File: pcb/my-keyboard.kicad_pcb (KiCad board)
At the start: 2 copper layers, 8 parts, among them J1 Conn_01x04_Socket, SW1 SW_Push, SW2 SW_Push, SW3 SW_Push, SW4 SW_Push, SW5 RotaryEncoder_Switch, SW6 RotaryEncoder_Switch, U1 MOUDLE-SEEEDUINO-XIAO

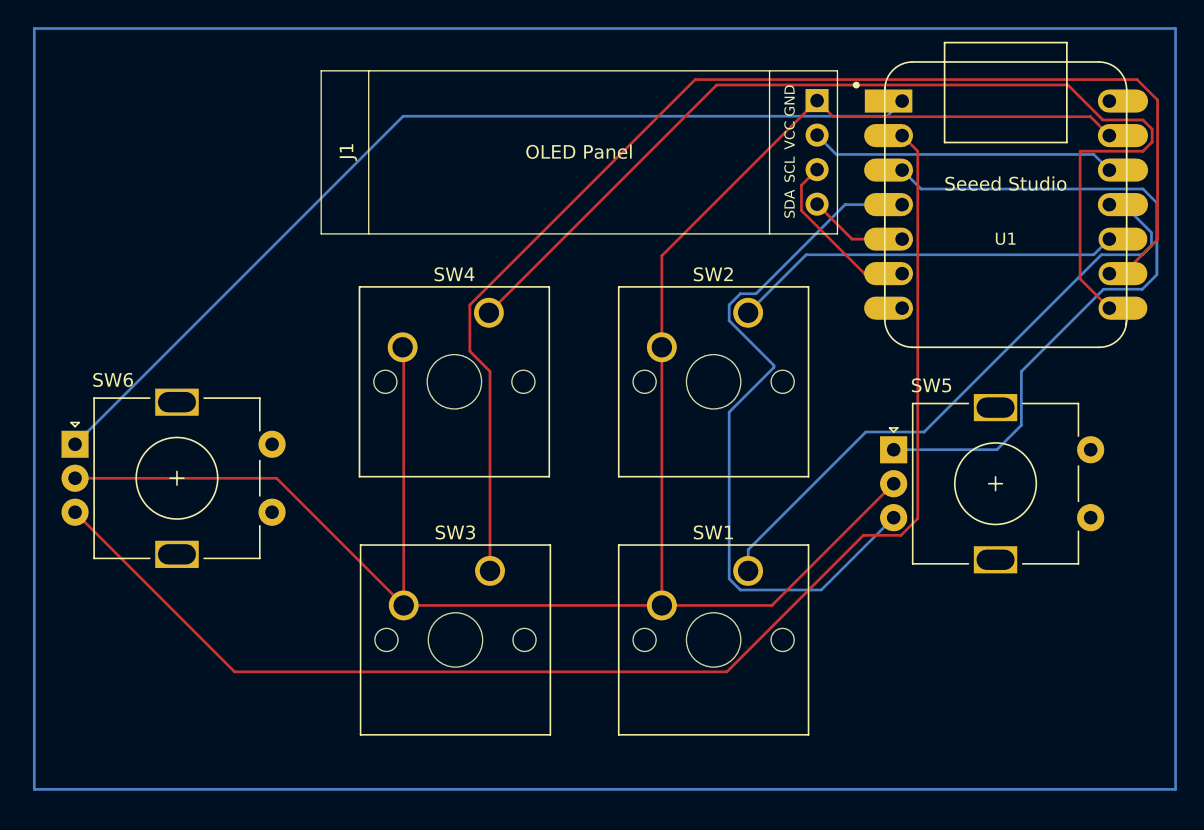
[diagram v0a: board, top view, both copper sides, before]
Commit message: New PCB and gerber files
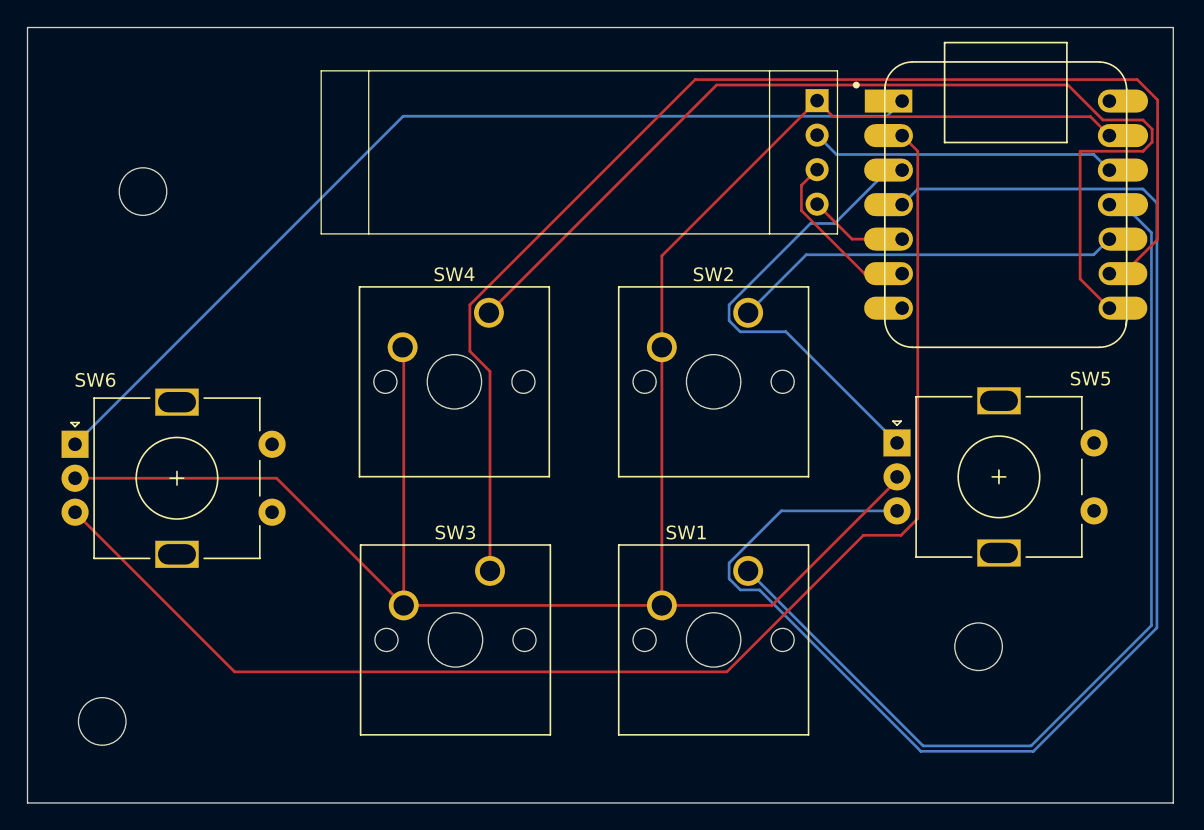
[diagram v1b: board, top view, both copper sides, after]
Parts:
- added H1: MountingHole, MountingHole:MountingHole_3.5mm, F.Cu at (167.0, 98.5)
- added H2: MountingHole, MountingHole:MountingHole_3.5mm, F.Cu at (105.5, 65.0)
- added H3: MountingHole, MountingHole:MountingHole_3.5mm, F.Cu at (102.5, 104.0)
- moved SW5 0.56 mm to (161.0, 83.5)
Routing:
- net Net-(U1-PA11_A3_D3): track 53.3 -> 106.5 mm
- net Net-(U1-PA6_A10_D10_MOSI): track 45.4 -> 70.5 mm
- net Net-(U1-PA10_A2_D2): track 52.1 -> 33.1 mm
- net Net-(U1-PA7_A8_D8_SCK): track 93.2 -> 92.1 mm
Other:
- board outline added: 84.3 x 57.1 mm
- board text added: "Controller PCB by Antoni Borowski"
